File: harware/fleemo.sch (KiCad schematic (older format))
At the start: 20 parts, among them P1 CONN_01X02, Q1 Q_NJFET_GDS

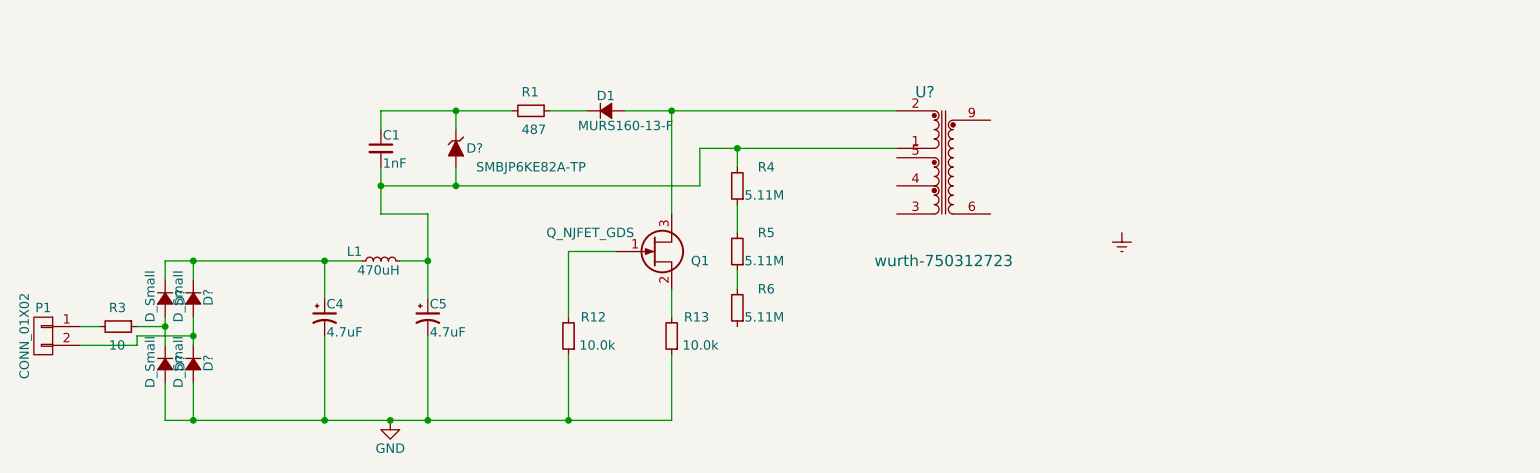
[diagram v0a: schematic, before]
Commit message: finish powe section
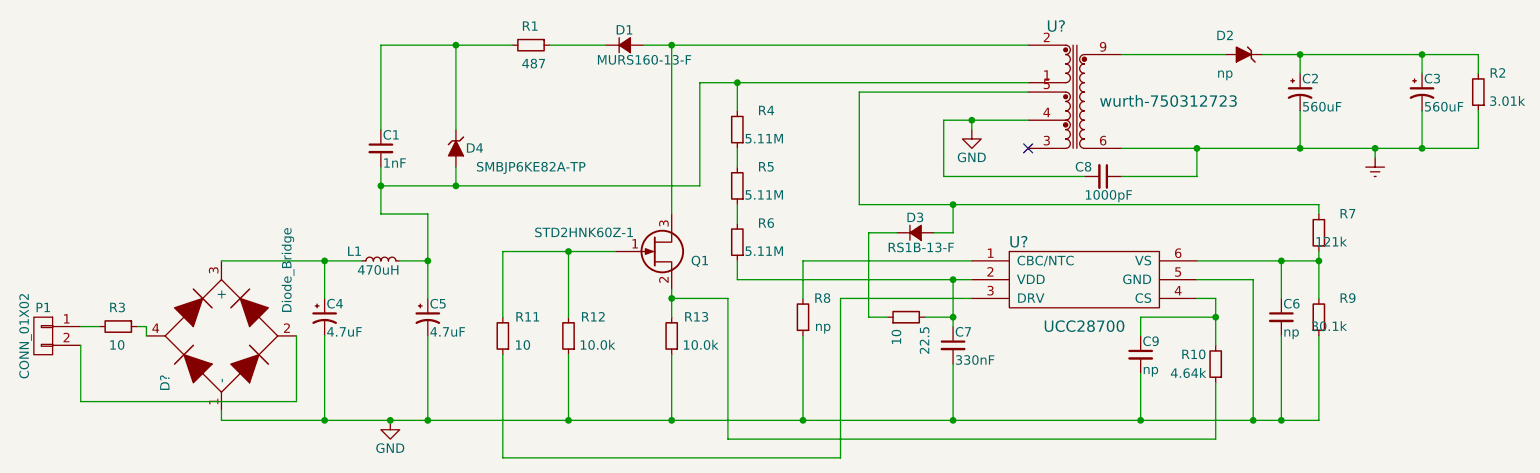
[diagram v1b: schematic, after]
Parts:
- removed D? (x4): D_Small, symbol D_Small
- added 22.5, R11: 10, symbol R_Small
- added C2, C3: 560uF, symbol CP1_Small
- added C6, C9: np, symbol C_Small
- added C7: 330nF, symbol C_Small
- added C8: 1000pF, symbol C_Small
- added D2: np, symbol ZENERsmall
- added D3: RS1B-13-F, symbol D_Small
- added D?: Diode_Bridge, symbol Diode_Bridge
- added R10: 4.64k, symbol R_Small
- added R2: 3.01k, symbol R_Small
- added R7: 121k, symbol R_Small
- added R8: np, symbol R_Small
- added R9: 30.1k, symbol R_Small
- added U?: UCC28700, symbol UCC28700
- Q1: value Q_NJFET_GDS -> STD2HNK60Z-1
- gave numbers to parts that had none: 1
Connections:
- net Earth: now also U?.6, C2.2, C3.2, C8.1, R2.1
- net GND: now also U?.4, C6.2, C7.2, C8.2, C9.2, D?.1 (-), R8.1, R9.1, U?.5 (GND)
- net at P1.2 (P2): now also D?.2
- net at C4.1, L1.1: now also D?.3 (+)
- net at Q1.1 (G), R12.2: now also R11.2
- net at Q1.2 (D), R13.2: now also R10.1
- net at U?.5: now also D3.2 (A), R7.2
- net at U?.9: now also D2.2 (A)
- net at R3.1: now also D?.4
- net at R6.1: now also 22.5.2, C7.1, U?.2 (VDD)
- new net: R8.2, U?.1 (CBC/NTC)
- new net: R11.1, U?.3 (DRV)
- new net: C9.1, R10.2, U?.4 (CS)
- new net: C6.1, R7.1, R9.2, U?.6 (VS)
- new net: 22.5.1, D3.1 (K)
- new net: C2.1, C3.1, D2.1 (K), R2.2
- no-connect marks 0 -> 1
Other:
- moved on the sheet: D1, R1, R4, R5, R6, U?
